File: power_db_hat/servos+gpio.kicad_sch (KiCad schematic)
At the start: 17 parts, among them J1 Conn_01x02_Pin, J11 Conn_01x03_Pin, J12 Conn_01x03_Pin, J15 Screw_Terminal_01x02, J4 Screw_Terminal_01x02, J6 Conn_01x02_Pin, K1 Relay_DPDT, K2 Relay_DPDT, U2 LDD-700LS, U6 LDD-700LS

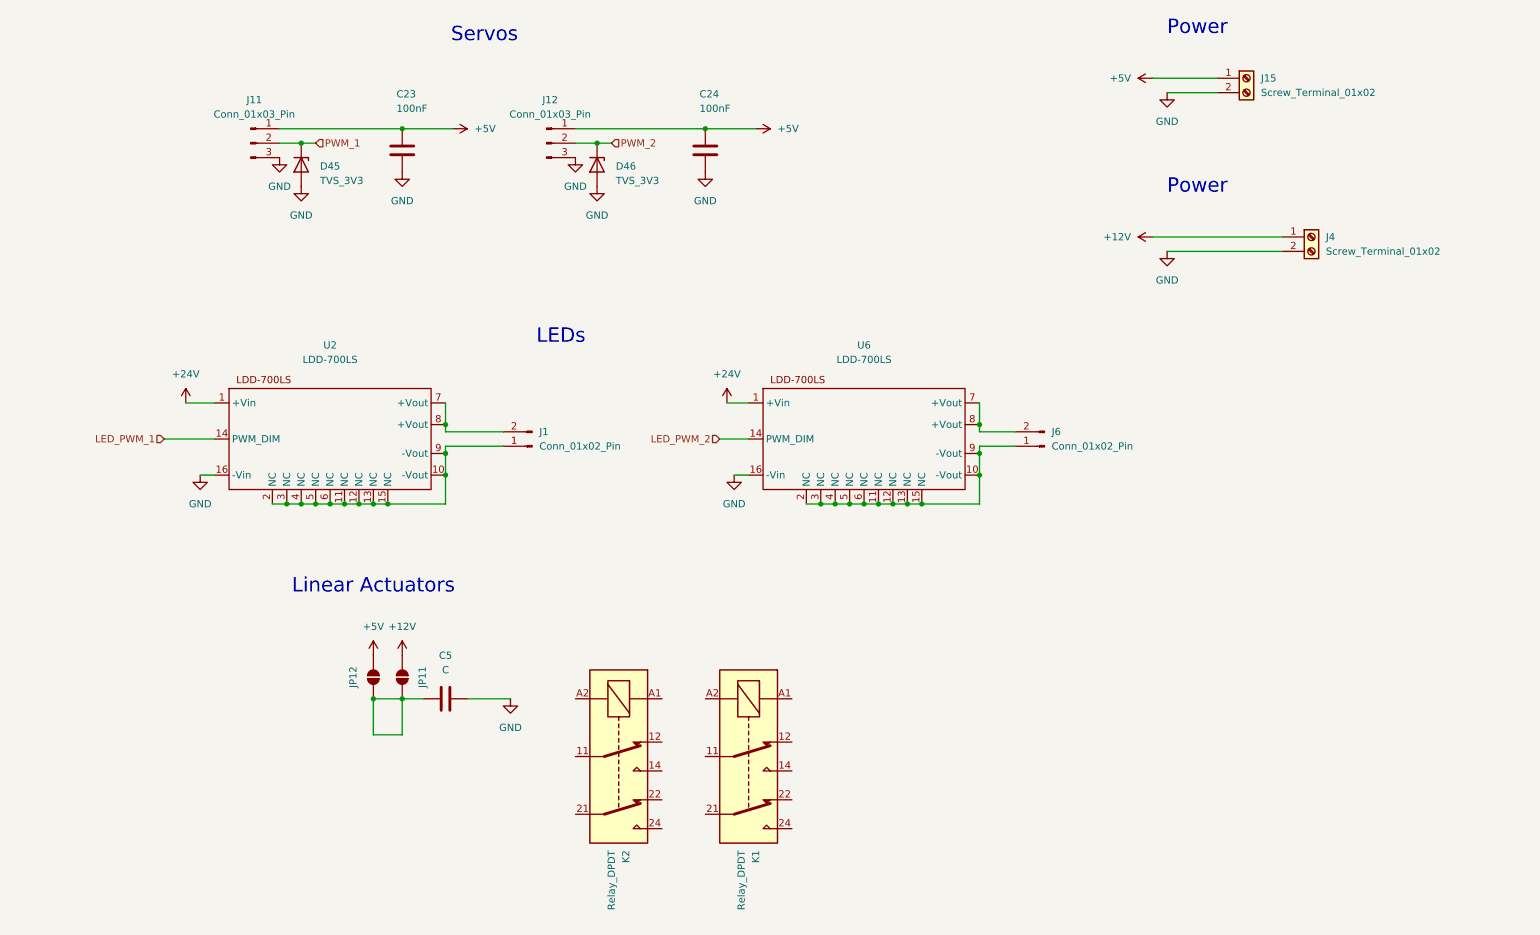
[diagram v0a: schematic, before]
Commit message: update
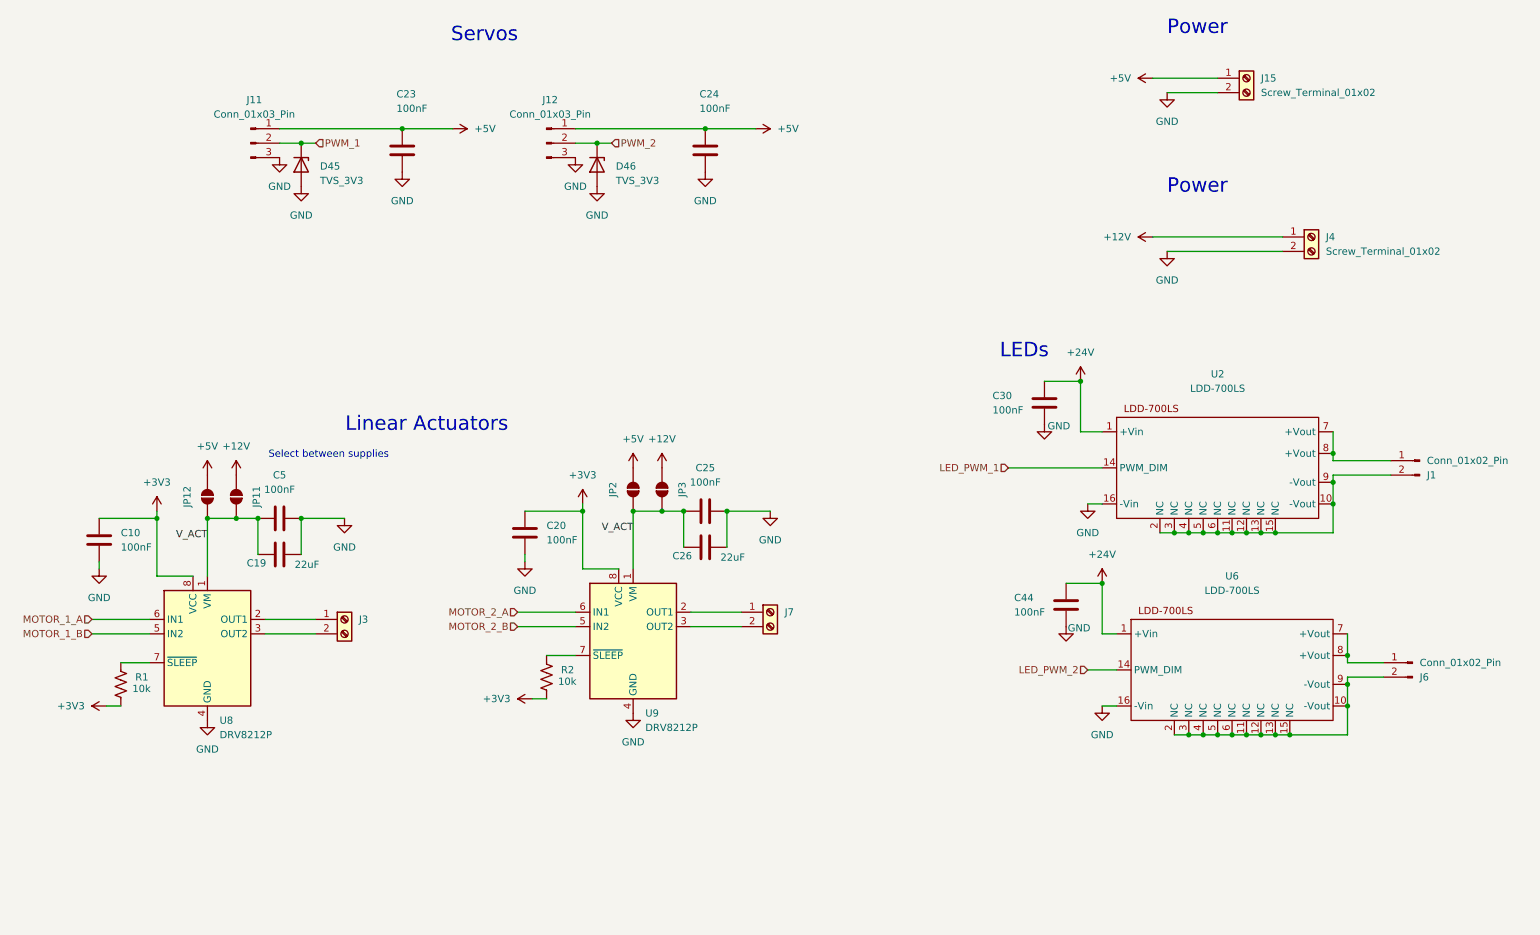
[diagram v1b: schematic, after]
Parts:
- removed K1, K2: Relay_DPDT, symbol Relay:Relay_DPDT
- added C10, C20, C25, C30, C44: 100nF, Capacitor_SMD:C_0603_1608Metric_Pad1.08x0.95mm_HandSolder, symbol Device:C
- added C19, C26: 22uF, Capacitor_SMD:C_0603_1608Metric_Pad1.08x0.95mm_HandSolder, symbol Device:C
- added J3, J7: Screw_Terminal_01x02, TerminalBlock:TerminalBlock_Xinya_XY308-2.54-2P_1x02_P2.54mm_Horizontal, symbol Connector:Screw_Terminal_01x02
- added JP2, JP3: SolderJumper_2_Open, Jumper:SolderJumper-2_P1.3mm_Open_TrianglePad1.0x1.5mm, symbol Jumper:SolderJumper_2_Open
- added R1, R2: 10k, Resistor_SMD:R_0603_1608Metric_Pad0.98x0.95mm_HandSolder, symbol Device:R_US
- added U8, U9: DRV8212P, Package_SON:WSON-8-1EP_2x2mm_P0.5mm_EP0.9x1.6mm_ThermalVias, symbol Driver_Motor:DRV8212P
- C5: value C -> 100nF; footprint (none) -> Capacitor_SMD:C_0603_1608Metric_Pad1.08x0.95mm_HandSolder
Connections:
- net +12V: now also JP3.1 (A)
- net +24V: now also C30.2, C44.2
- net +5V: now also JP2.2 (B)
- net GND: now also C10.2, C19.2, C20.2, C25.2, C26.2, C30.1, C44.1, U8.4 (GND), U8.9 (GND), U9.4 (GND), U9.9 (GND)
- net V_ACT: now reaches C5.1, JP11.2 (B), JP12.1 (A)
- net V_ACT: now also C19.1, C25.1, C26.1, JP2.1 (A), JP3.2 (B), U8.1 (VM), U9.1 (VM)
- net at U2.10 (-Vout), U2.11 (NC), U2.12 (NC)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: now also J1.2 (Pin_2); no longer J1.1 (Pin_1)
- net at U2.7 (+Vout), U2.8 (+Vout): now also J1.1 (Pin_1); no longer J1.2 (Pin_2)
- net at U6.10 (-Vout), U6.11 (NC), U6.12 (NC)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: now also J6.2 (Pin_2); no longer J6.1 (Pin_1)
- net at U6.7 (+Vout), U6.8 (+Vout): now also J6.1 (Pin_1); no longer J6.2 (Pin_2)
- new net: R2.1, U9.7 (~{SLEEP})
- new net: J3.1 (Pin_1), U8.2 (OUT1)
- new net: J3.2 (Pin_2), U8.3 (OUT2)
- new net: R1.1, U8.7 (~{SLEEP})
- new net: J7.1 (Pin_1), U9.2 (OUT1)
- new net: J7.2 (Pin_2), U9.3 (OUT2)
- new net +3V3: C10.1, C20.1, R1.2, R2.2, U8.8 (VCC), U9.8 (VCC)
- new net MOTOR_1_A: U8.6 (IN1)
- new net MOTOR_1_B: U8.5 (IN2)
- new net MOTOR_2_A: U9.6 (IN1)
- new net MOTOR_2_B: U9.5 (IN2)
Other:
- note added: "Select between supplies"
- moved on the sheet: C5, J1, J6, JP11, JP12, U2, U6
